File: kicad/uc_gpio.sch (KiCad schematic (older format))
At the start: 1 part, among them U301 TMS320F28388DZWTS

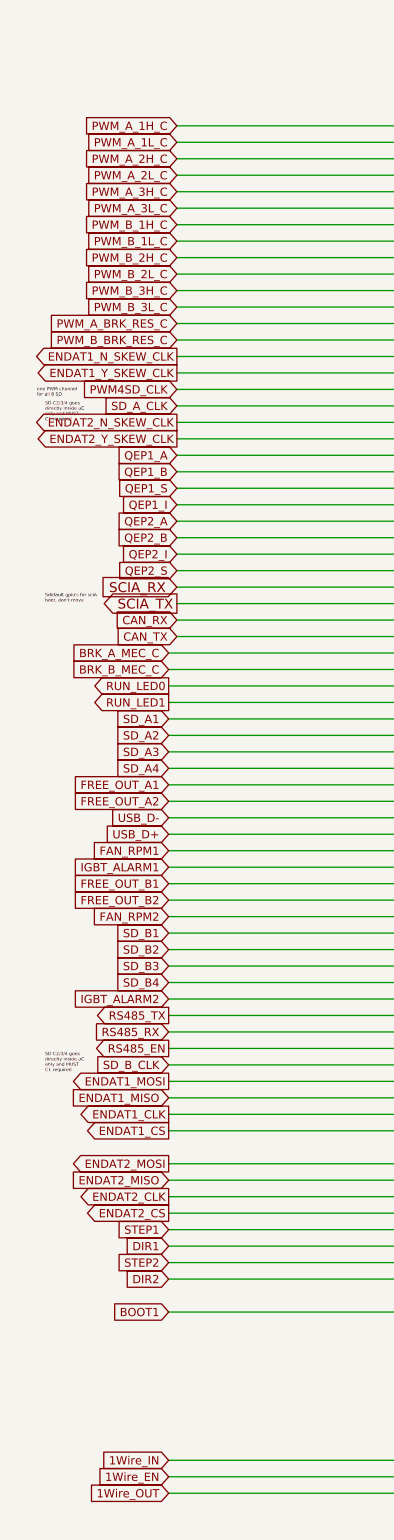
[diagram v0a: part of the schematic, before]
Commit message: beginine routing... far far away
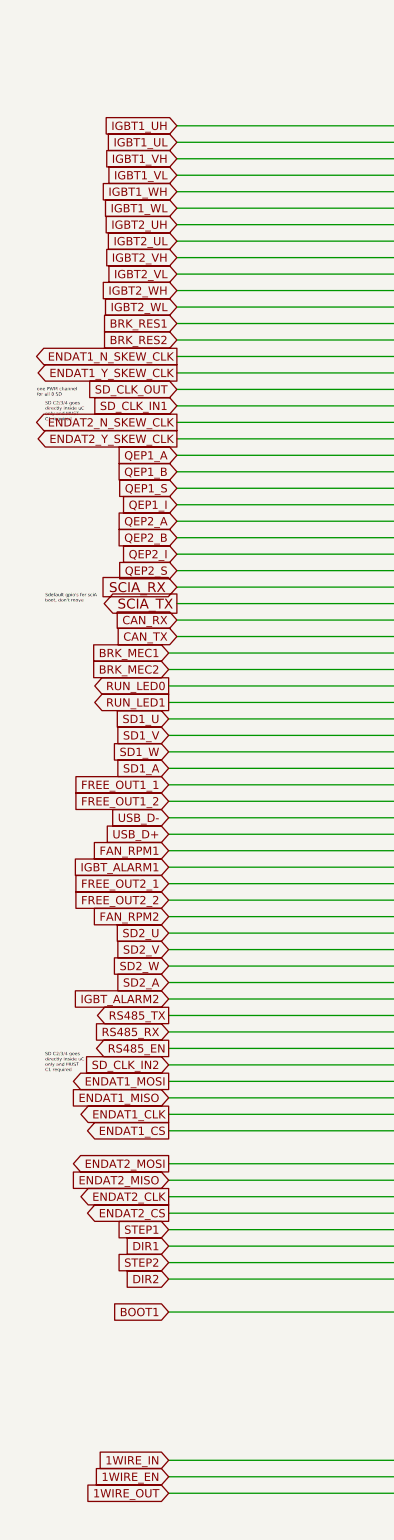
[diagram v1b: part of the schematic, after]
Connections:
- net 1Wire_EN renamed 1WIRE_EN
- net 1Wire_IN renamed 1WIRE_IN
- net 1Wire_OUT renamed 1WIRE_OUT
- net BRK_A_MEC_C renamed BRK_MEC1
- net BRK_B_MEC_C renamed BRK_MEC2
- net FREE_OUT_A1 renamed FREE_OUT1_1
- net FREE_OUT_A2 renamed FREE_OUT1_2
- net FREE_OUT_B1 renamed FREE_OUT2_1
- net FREE_OUT_B2 renamed FREE_OUT2_2
- net PWM4SD_CLK renamed SD_CLK_OUT
- net PWM_A_1H_C renamed IGBT1_UH
- net PWM_A_1L_C renamed IGBT1_UL
- net PWM_A_2H_C renamed IGBT1_VH
- net PWM_A_2L_C renamed IGBT1_VL
- net PWM_A_3H_C renamed IGBT1_WH
- net PWM_A_3L_C renamed IGBT1_WL
- net PWM_A_BRK_RES_C renamed BRK_RES1
- net PWM_B_1H_C renamed IGBT2_UH
- net PWM_B_1L_C renamed IGBT2_UL
- net PWM_B_2H_C renamed IGBT2_VH
- net PWM_B_2L_C renamed IGBT2_VL
- net PWM_B_3H_C renamed IGBT2_WH
- net PWM_B_3L_C renamed IGBT2_WL
- net PWM_B_BRK_RES_C renamed BRK_RES2
- net SD_A1 renamed SD1_U
- net SD_A2 renamed SD1_V
- net SD_A3 renamed SD1_W
- net SD_A4 renamed SD1_A
- net SD_A_CLK renamed SD_CLK_IN1
- net SD_B1 renamed SD2_U
- net SD_B2 renamed SD2_V
- net SD_B3 renamed SD2_W
- net SD_B4 renamed SD2_A
- net SD_B_CLK renamed SD_CLK_IN2
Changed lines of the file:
@@
 Wire Wire Line
 	3150 10200 4800 10200
-Text GLabel 3200 2100 0    50   Input ~ 0
-PWM_A_1H_C
-Text GLabel 3200 2300 0    50   Input ~ 0
-PWM_A_2H_C
-Text GLabel 3200 2500 0    50   Input ~ 0
-PWM_A_3H_C
-Text GLabel 3200 2200 0    50   Input ~ 0
-PWM_A_1L_C
-Text GLabel 3200 2400 0    50   Input ~ 0
-PWM_A_2L_C
-Text GLabel 3200 2600 0    50   Input ~ 0
-PWM_A_3L_C
-Text GLabel 3200 2900 0    50   Input ~ 0
-PWM_B_2H_C
-Text GLabel 3200 2700 0    50   Input ~ 0
-PWM_B_1H_C
-Text GLabel 3200 2800 0    50   Input ~ 0
-PWM_B_1L_C
-Text GLabel 3200 3100 0    50   Input ~ 0
-PWM_B_3H_C
-Text GLabel 3200 3200 0    50   Input ~ 0
-PWM_B_3L_C
-Text GLabel 3200 3000 0    50   Input ~ 0
-PWM_B_2L_C
 Wire Wire Line
 	3150 5500 4800 5500
@@
 Wire Wire Line
 	3200 5000 4800 5000
-Text GLabel 3150 5700 0    50   Input ~ 0
-SD_A1
-Text GLabel 3150 5800 0    50   Input ~ 0
-SD_A2
-Text GLabel 3150 5900 0    50   Input ~ 0
-SD_A3
-Text GLabel 3150 6000 0    50   Input ~ 0
-SD_A4
-Text GLabel 3200 3300 0    50   Input ~ 0
-PWM_A_BRK_RES_C
-Text GLabel 3200 3400 0    50   Input ~ 0
-PWM_B_BRK_RES_C
-Text GLabel 3150 7000 0    50   Input ~ 0
-SD_B1
-Text GLabel 3150 7100 0    50   Input ~ 0
-SD_B2
-Text GLabel 3150 7200 0    50   Input ~ 0
-SD_B3
 Wire Wire Line
 	3150 7000 4800 7000
@@
 Wire Wire Line
 	3200 3800 4800 3800
-Text GLabel 3200 3800 0    50   Input ~ 0
-SD_A_CLK
 Text GLabel 3200 3700 0    50   Input ~ 0
-PWM4SD_CLK
+SD_CLK_OUT
 Wire Wire Line
 	3200 3700 4800 3700
@@
 Text Notes 2400 7850 0    20   ~ 0
 SD C2/3/4 goes\ndirectly inside uC\nonly and MUST  \nC1 required
-Text GLabel 3150 7800 0    50   Input ~ 0
-SD_B_CLK
 Wire Wire Line
 	3150 7300 4800 7300
-Text GLabel 3150 7300 0    50   Input ~ 0
-SD_B4
 Text GLabel 3150 7600 0    50   Input ~ 0
 RS485_RX
@@
 Wire Wire Line
 	8350 2600 9700 2600
-Text GLabel 3150 6100 0    50   Input ~ 0
-FREE_OUT_A1
-Text GLabel 3150 6200 0    50   Input ~ 0
-FREE_OUT_A2
-Text GLabel 3150 6700 0    50   Input ~ 0
-FREE_OUT_B1
-Text GLabel 3150 6800 0    50   Input ~ 0
-FREE_OUT_B2
 Wire Wire Line
 	3200 2100 4800 2100
-Text GLabel 3150 5400 0    50   Input ~ 0
-BRK_B_MEC_C
-Text GLabel 3150 5300 0    50   Input ~ 0
-BRK_A_MEC_C
 Wire Wire Line
 	3150 5300 4800 5300
@@
 	8350 9600 9700 9600
 Text GLabel 3150 10400 0    50   Input ~ 0
-1Wire_OUT
+1WIRE_OUT
 Text GLabel 3150 10200 0    50   Input ~ 0
-1Wire_IN
+1WIRE_IN
 Text GLabel 3150 10300 0    50   Input ~ 0
-1Wire_EN
+1WIRE_EN
 NoConn ~ 4800 9200
 NoConn ~ 4800 9400
@@
 Wire Wire Line
 	4800 7700 3150 7700
-Text GLabel 3150 6900 0    50   Input ~ 0
-FAN_RPM2
-Text GLabel 3150 7400 0    50   Input ~ 0
-IGBT_ALARM2
-Text GLabel 3150 6500 0    50   Input ~ 0
-FAN_RPM1
-Text GLabel 3150 6600 0    50   Input ~ 0
-IGBT_ALARM1
 Text GLabel 3150 8800 0    50   Input ~ 0
 STEP1
@@
 Text GLabel 9700 8900 2    50   Input ~ 0
 ECAT_MDCLK
+Text GLabel 3200 3400 0    50   Input ~ 0
+BRK_RES2
+Text GLabel 3150 6800 0    50   Input ~ 0
+FREE_OUT2_2
+Text GLabel 3150 6900 0    50   Input ~ 0
+FAN_RPM2
+Text GLabel 3150 5400 0    50   Input ~ 0
+BRK_MEC2
+Text GLabel 3150 6700 0    50   Input ~ 0
+FREE_OUT2_1
+Text GLabel 3150 7400 0    50   Input ~ 0
+IGBT_ALARM2
+Text GLabel 3200 3300 0    50   Input ~ 0
+BRK_RES1
+Text GLabel 3150 6200 0    50   Input ~ 0
+FREE_OUT1_2
+Text GLabel 3150 6500 0    50   Input ~ 0
+FAN_RPM1
+Text GLabel 3150 5300 0    50   Input ~ 0
+BRK_MEC1
+Text GLabel 3150 6100 0    50   Input ~ 0
+FREE_OUT1_1
+Text GLabel 3150 6600 0    50   Input ~ 0
+IGBT_ALARM1
+Text GLabel 3200 2100 0    50   Input ~ 0
+IGBT1_UH
+Text GLabel 3200 2200 0    50   Input ~ 0
+IGBT1_UL
+Text GLabel 3200 2300 0    50   Input ~ 0
+IGBT1_VH
+Text GLabel 3200 2400 0    50   Input ~ 0
+IGBT1_VL
+Text GLabel 3200 2500 0    50   Input ~ 0
+IGBT1_WH
+Text GLabel 3200 2600 0    50   Input ~ 0
+IGBT1_WL
+Text GLabel 3200 2700 0    50   Input ~ 0
+IGBT2_UH
+Text GLabel 3200 2800 0    50   Input ~ 0
+IGBT2_UL
+Text GLabel 3200 2900 0    50   Input ~ 0
+IGBT2_VH
+Text GLabel 3200 3000 0    50   Input ~ 0
+IGBT2_VL
+Text GLabel 3200 3100 0    50   Input ~ 0
+IGBT2_WH
+Text GLabel 3200 3200 0    50   Input ~ 0
+IGBT2_WL
+Text GLabel 3200 3800 0    50   Input ~ 0
+SD_CLK_IN1
+Text GLabel 3150 5700 0    50   Input ~ 0
+SD1_U
+Text GLabel 3150 5800 0    50   Input ~ 0
+SD1_V
+Text GLabel 3150 5900 0    50   Input ~ 0
+SD1_W
+Text GLabel 3150 6000 0    50   Input ~ 0
+SD1_A
+Text GLabel 3150 7800 0    50   Input ~ 0
+SD_CLK_IN2
+Text GLabel 3150 7000 0    50   Input ~ 0
+SD2_U
+Text GLabel 3150 7100 0    50   Input ~ 0
+SD2_V
+Text GLabel 3150 7200 0    50   Input ~ 0
+SD2_W
+Text GLabel 3150 7300 0    50   Input ~ 0
+SD2_A
 $EndSCHEMATC
